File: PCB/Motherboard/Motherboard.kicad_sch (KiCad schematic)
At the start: 12 parts, among them J1 Conn_01x03_Socket, J10 Screw_Terminal_01x02, J2 Screw_Terminal_01x02, J3 Screw_Terminal_01x02, J4 Screw_Terminal_01x02, J5 Screw_Terminal_01x02, J6 Screw_Terminal_01x02, J7 Screw_Terminal_01x02, J8 Screw_Terminal_01x02, J9 Screw_Terminal_01x02

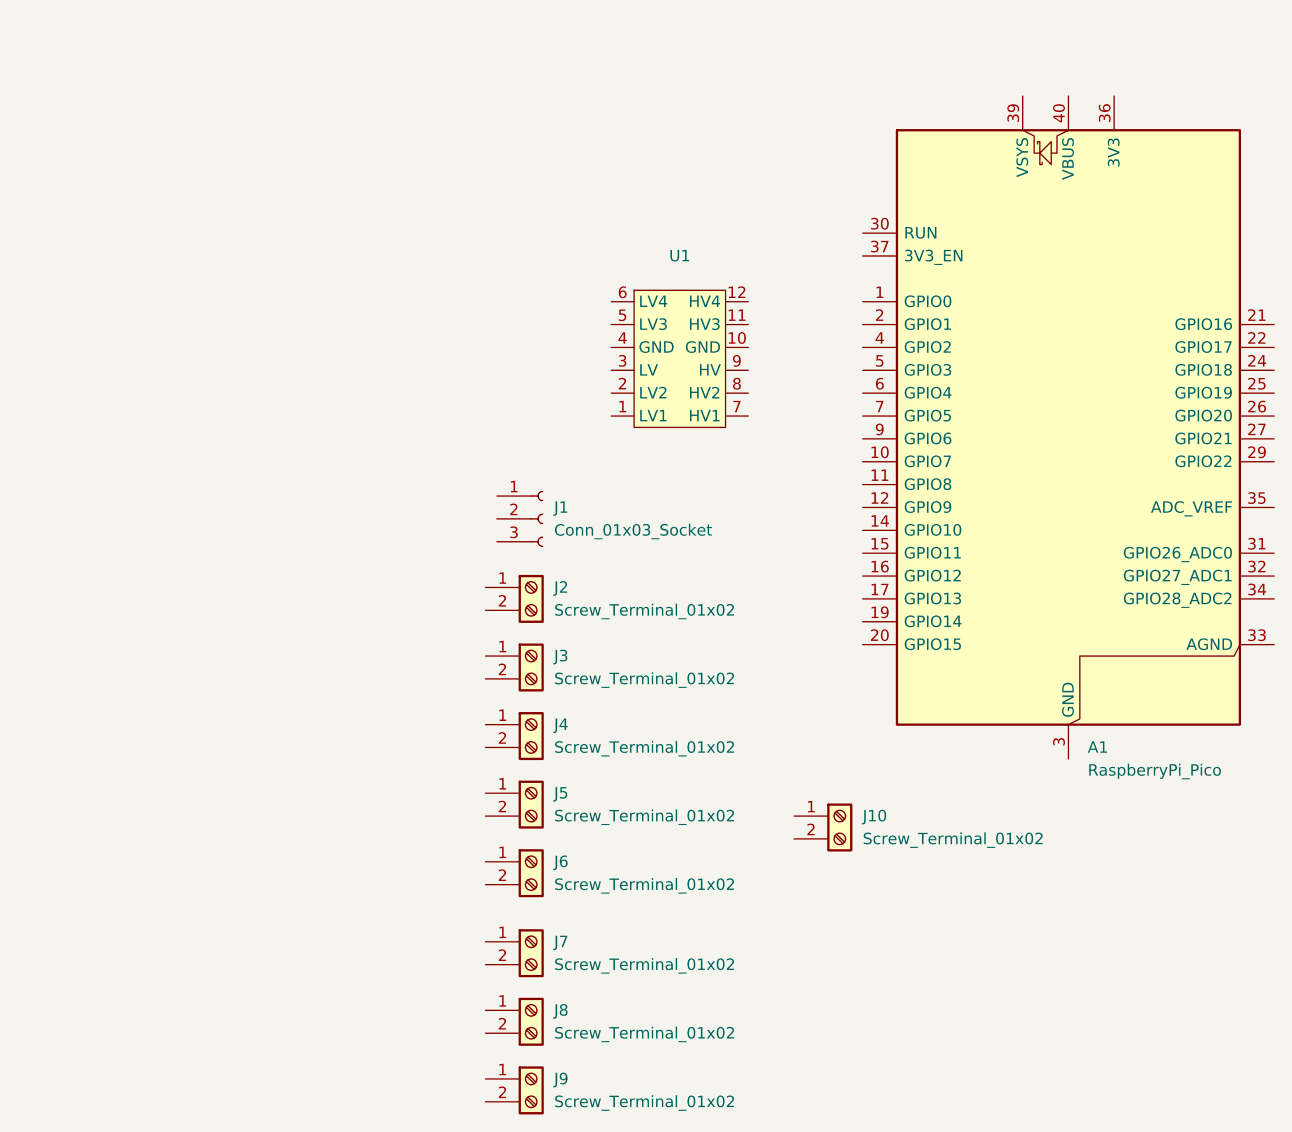
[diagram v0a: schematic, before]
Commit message: custom footprints and general layout
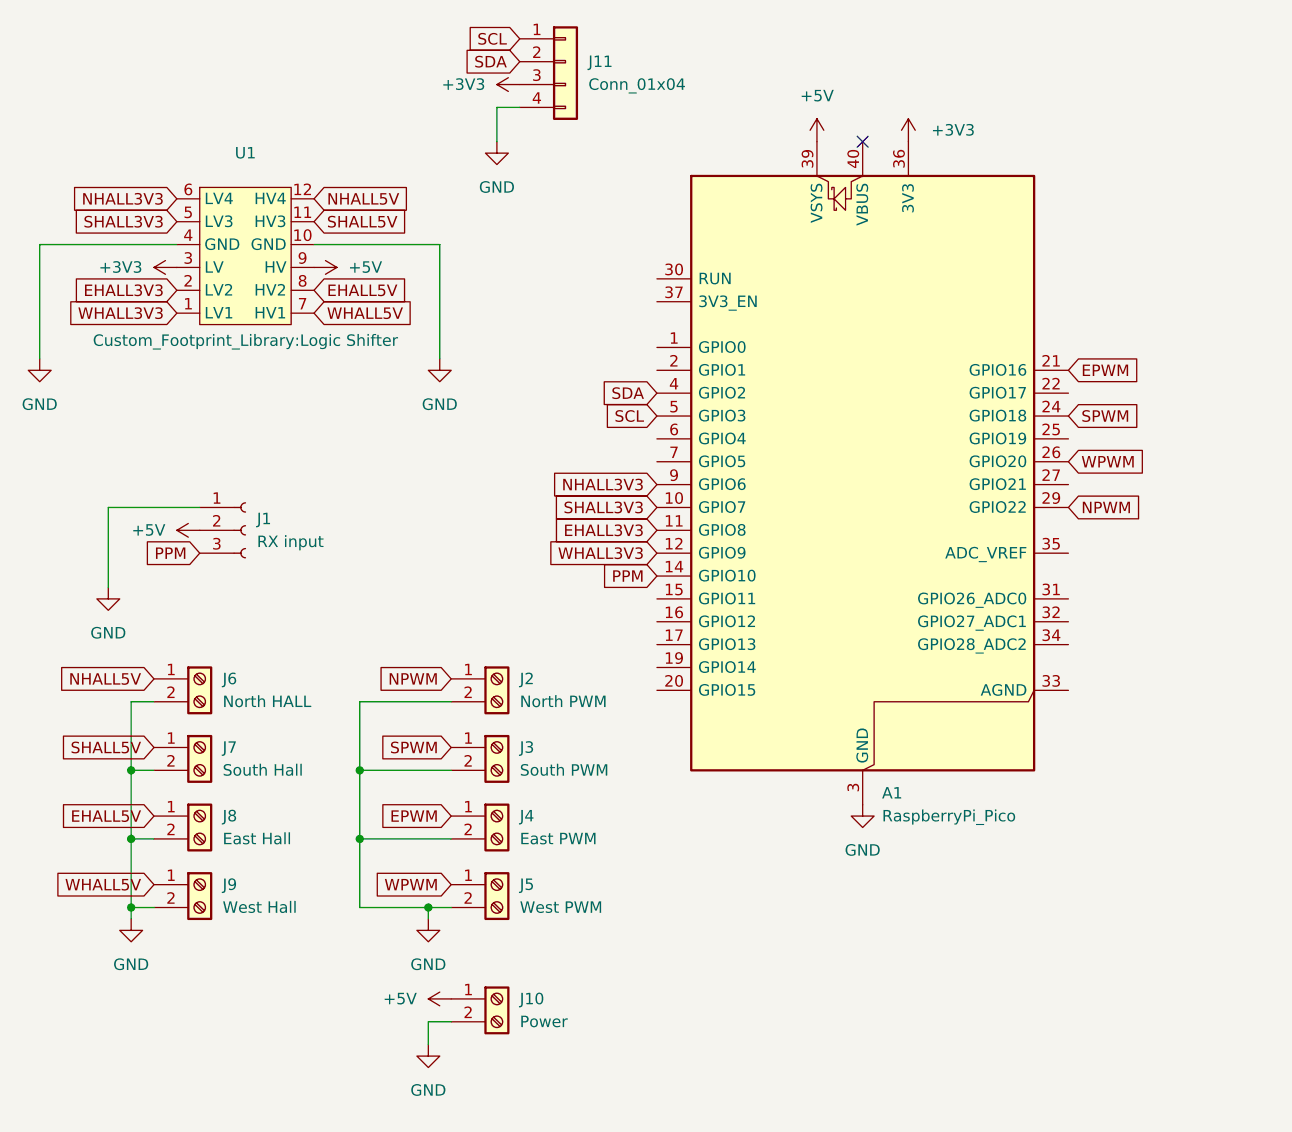
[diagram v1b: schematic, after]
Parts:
- added J11: Conn_01x04, Connector_JST:JST_PH_B4B-PH-K_1x04_P2.00mm_Vertical, symbol Connector_Generic:Conn_01x04
- J1: value Conn_01x03_Socket -> RX input; footprint Connector_PinSocket_2.54mm:PinSocket_1x03_P2.54mm_Vertical -> Connector_PinHeader_2.54mm:PinHeader_1x03_P2.54mm_Vertical
- J10: value Screw_Terminal_01x02 -> Power
- J2: value Screw_Terminal_01x02 -> North PWM
- J3: value Screw_Terminal_01x02 -> South PWM
- J4: value Screw_Terminal_01x02 -> East PWM
- J5: value Screw_Terminal_01x02 -> West PWM
- J6: value Screw_Terminal_01x02 -> North HALL
- J7: value Screw_Terminal_01x02 -> South Hall
- J8: value Screw_Terminal_01x02 -> East Hall
- J9: value Screw_Terminal_01x02 -> West Hall
- U1: footprint (none) -> Custom_Footprint_Library:Logic Shifter
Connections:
- net WHALL3V3: now reaches U1.1 (LV1)
- net WHALL3V3: now also A1.12 (GPIO9)
- net GND: now reaches U1.10 (GND)
- net GND: now also A1.13 (GND), A1.18 (GND), A1.23 (GND), A1.28 (GND), A1.3 (GND), A1.38 (GND), A1.8 (GND), J1.1 (Pin_1), J10.2 (Pin_2), J2.2 (Pin_2), J3.2 (Pin_2), J4.2 (Pin_2), J5.2 (Pin_2), J6.2 (Pin_2), J7.2 (Pin_2), J8.2 (Pin_2), J9.2 (Pin_2), U1.4 (GND), J11.4 (Pin_4)
- net SHALL5V: now reaches U1.11 (HV3)
- net SHALL5V: now also J7.1 (Pin_1)
- net NHALL5V: now reaches U1.12 (HV4)
- net NHALL5V: now also J6.1 (Pin_1)
- net EHALL3V3: now reaches U1.2 (LV2)
- net EHALL3V3: now also A1.11 (GPIO8)
- net +3V3: now reaches U1.3 (LV)
- net +3V3: now also A1.36 (3V3), J11.3 (Pin_3)
- net SHALL3V3: now reaches U1.5 (LV3)
- net SHALL3V3: now also A1.10 (GPIO7)
- net NHALL3V3: now reaches U1.6 (LV4)
- net NHALL3V3: now also A1.9 (GPIO6)
- net WHALL5V: now reaches U1.7 (HV1)
- net WHALL5V: now also J9.1 (Pin_1)
- net EHALL5V: now reaches U1.8 (HV2)
- net EHALL5V: now also J8.1 (Pin_1)
- net +5V: now reaches U1.9 (HV)
- net +5V: now also A1.39 (VSYS), J1.2 (Pin_2), J10.1 (Pin_1)
- net PPM: now reaches A1.14 (GPIO10)
- net PPM: now also J1.3 (Pin_3)
- net EPWM: now reaches A1.21 (GPIO16)
- net EPWM: now also J4.1 (Pin_1)
- net SPWM: now reaches A1.24 (GPIO18)
- net SPWM: now also J3.1 (Pin_1)
- net WPWM: now reaches A1.26 (GPIO20)
- net WPWM: now also J5.1 (Pin_1)
- net NPWM: now reaches A1.29 (GPIO22)
- net NPWM: now also J2.1 (Pin_1)
- net SDA: now reaches A1.4 (GPIO2)
- net SDA: now also J11.2 (Pin_2)
- net SCL: now reaches A1.5 (GPIO3)
- net SCL: now also J11.1 (Pin_1)
- no-connect marks 0 -> 1
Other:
- moved on the sheet: A1, J1, J10, J2, J3, J4, J5, J6, J7, J8, J9, U1
